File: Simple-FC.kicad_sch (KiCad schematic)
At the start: 2 parts, among them U1 RP2350A, U3 LSM6DSM

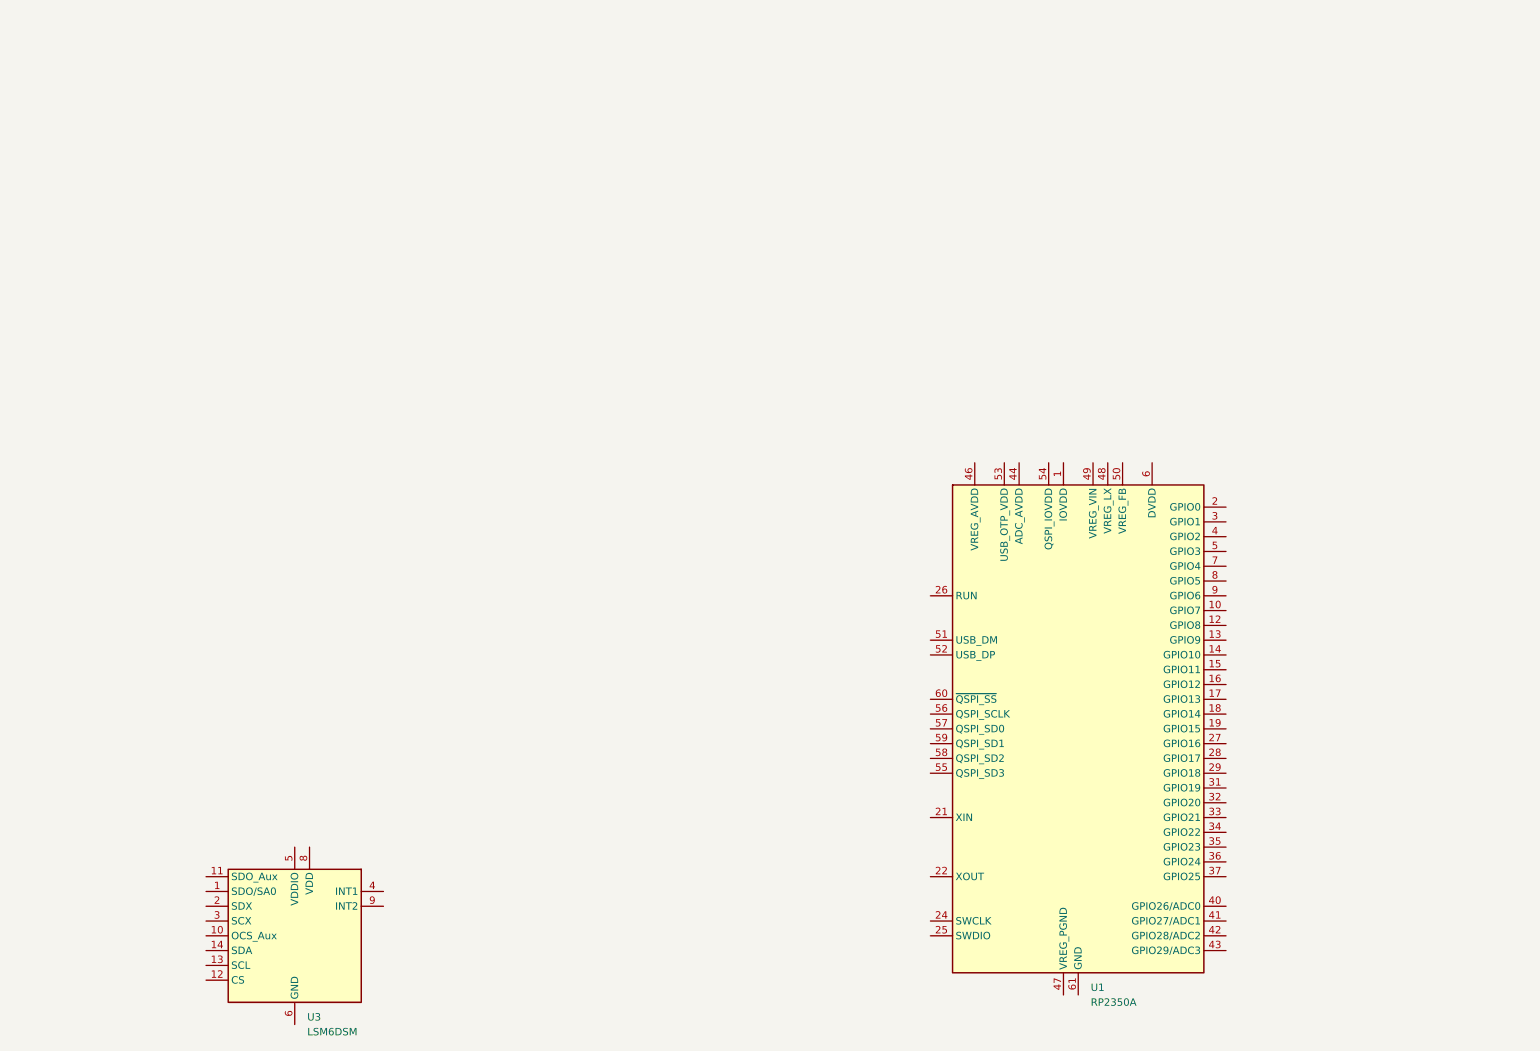
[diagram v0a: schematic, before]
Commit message: selected parts
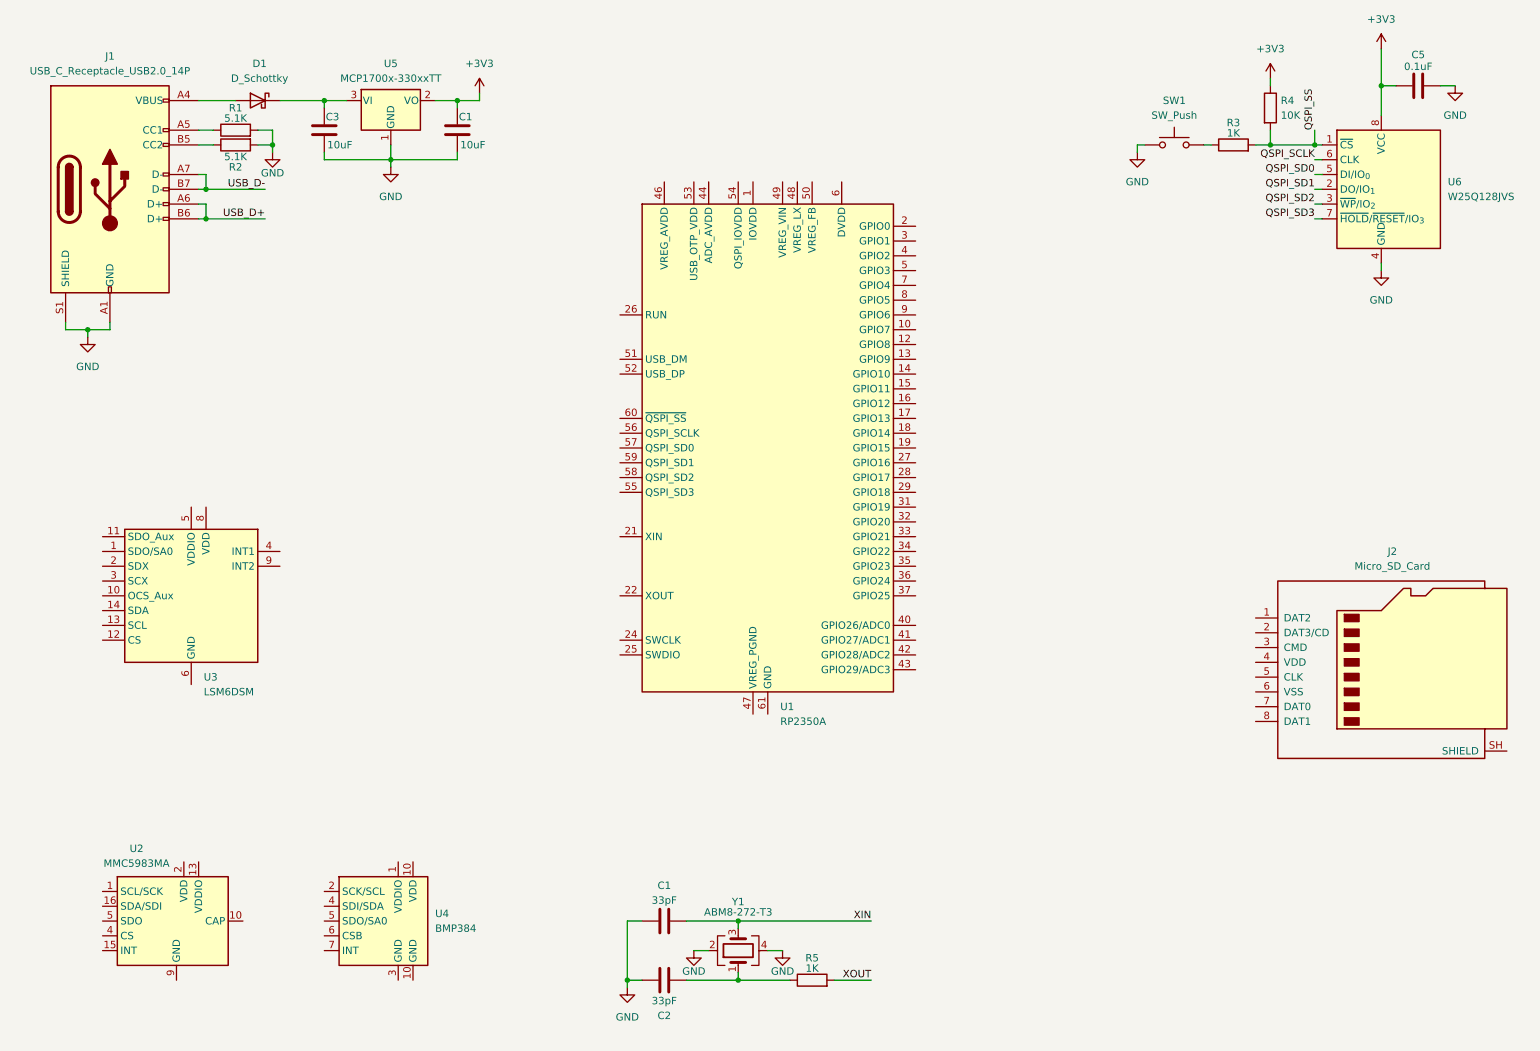
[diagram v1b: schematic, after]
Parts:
- added C1, C2: 33pF, Capacitor_SMD:C_0402_1005Metric, symbol Device:C
- added C1, C3: 10uF, Capacitor_SMD:C_0603_1608Metric, symbol Device:C
- added C5: 0.1uF, Capacitor_SMD:C_0402_1005Metric, symbol Device:C
- added D1: D_Schottky, Diode_SMD:D_0402_1005Metric, symbol Device:D_Schottky
- added J1: USB_C_Receptacle_USB2.0_14P, Connector_USB:USB_C_Receptacle_HRO_TYPE-C-31-M-12, symbol Connector:USB_C_Receptacle_USB2.0_14P
- added J2: Micro_SD_Card, Connector_Card:microSD_HC_Molex_47219-2001, symbol Connector:Micro_SD_Card
- added R1, R2: 5.1K, Resistor_SMD:R_0402_1005Metric, symbol Device:R
- added R3, R5: 1K, Resistor_SMD:R_0402_1005Metric, symbol Device:R
- added R4: 10K, Resistor_SMD:R_0402_1005Metric, symbol Device:R
- added SW1: SW_Push, Button_Switch_SMD:SW_Push_SPST_NO_Alps_SKRK, symbol Switch:SW_Push
- added U2: MMC5983MA, Package_LGA:LGA-16_3x3mm_P0.5mm, symbol Simple-FC:MMC5983MA
- added U4: BMP384, Package_LGA:ST_HLGA-10_2x2mm_P0.5mm_LayoutBorder3x2y, symbol Simple-FC:BMP384
- added U5: MCP1700x-330xxTT, Package_TO_SOT_SMD:SOT-23, symbol Regulator_Linear:MCP1700x-330xxTT
- added U6: W25Q128JVS, Package_SON:Winbond_USON-8-1EP_3x2mm_P0.5mm_EP0.2x1.6mm, symbol Memory_Flash:W25Q128JVS
- added Y1: ABM8-272-T3, Crystal:Crystal_SMD_3225-4Pin_3.2x2.5mm, symbol Device:Crystal_GND24
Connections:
- new net: C2.1, R5.1, Y1.1
- new net: J1.A5 (CC1), R1.1
- new net: D1.2 (A), J1.A4 (VBUS), J1.A9 (VBUS), J1.B4 (VBUS), J1.B9 (VBUS)
- new net: J1.B5 (CC2), R2.1
- new net: C3.1, D1.1 (K), U5.3 (VI)
- new net: R3.1, SW1.2
- new net +3V3: C1.1, C5.1, R4.1, U5.2 (VO), U6.8 (VCC)
- new net GND: C1.1, C1.2, C2.2, C3.2, C5.2, J1.A1 (GND), J1.A12 (GND), J1.B1 (GND), J1.B12 (GND), J1.S1 (SHIELD), R1.2, R2.2, SW1.1, U5.1 (GND), U6.4 (GND), Y1.2, Y1.4
- new net QSPI_SCLK: U6.6 (CLK)
- new net QSPI_SD0: U6.5 (DI/IO_{0})
- new net QSPI_SD1: U6.2 (DO/IO_{1})
- new net QSPI_SD2: U6.3 (~{WP}/IO_{2})
- new net QSPI_SD3: U6.7 (~{HOLD}/~{RESET}/IO_{3})
- new net QSPI_SS: R3.2, R4.2, U6.1 (~{CS})
- new net USB_D+: J1.A6 (D+), J1.B6 (D+)
- new net USB_D-: J1.A7 (D-), J1.B7 (D-)
- new net XIN: C1.2, Y1.3
- new net XOUT: R5.2
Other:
- moved on the sheet: U1, U3
